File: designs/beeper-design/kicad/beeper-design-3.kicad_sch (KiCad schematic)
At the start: 30 parts, among them U12 DRV2605YZFR, U13 CSD75207W15, U3 BQ51003YFPR

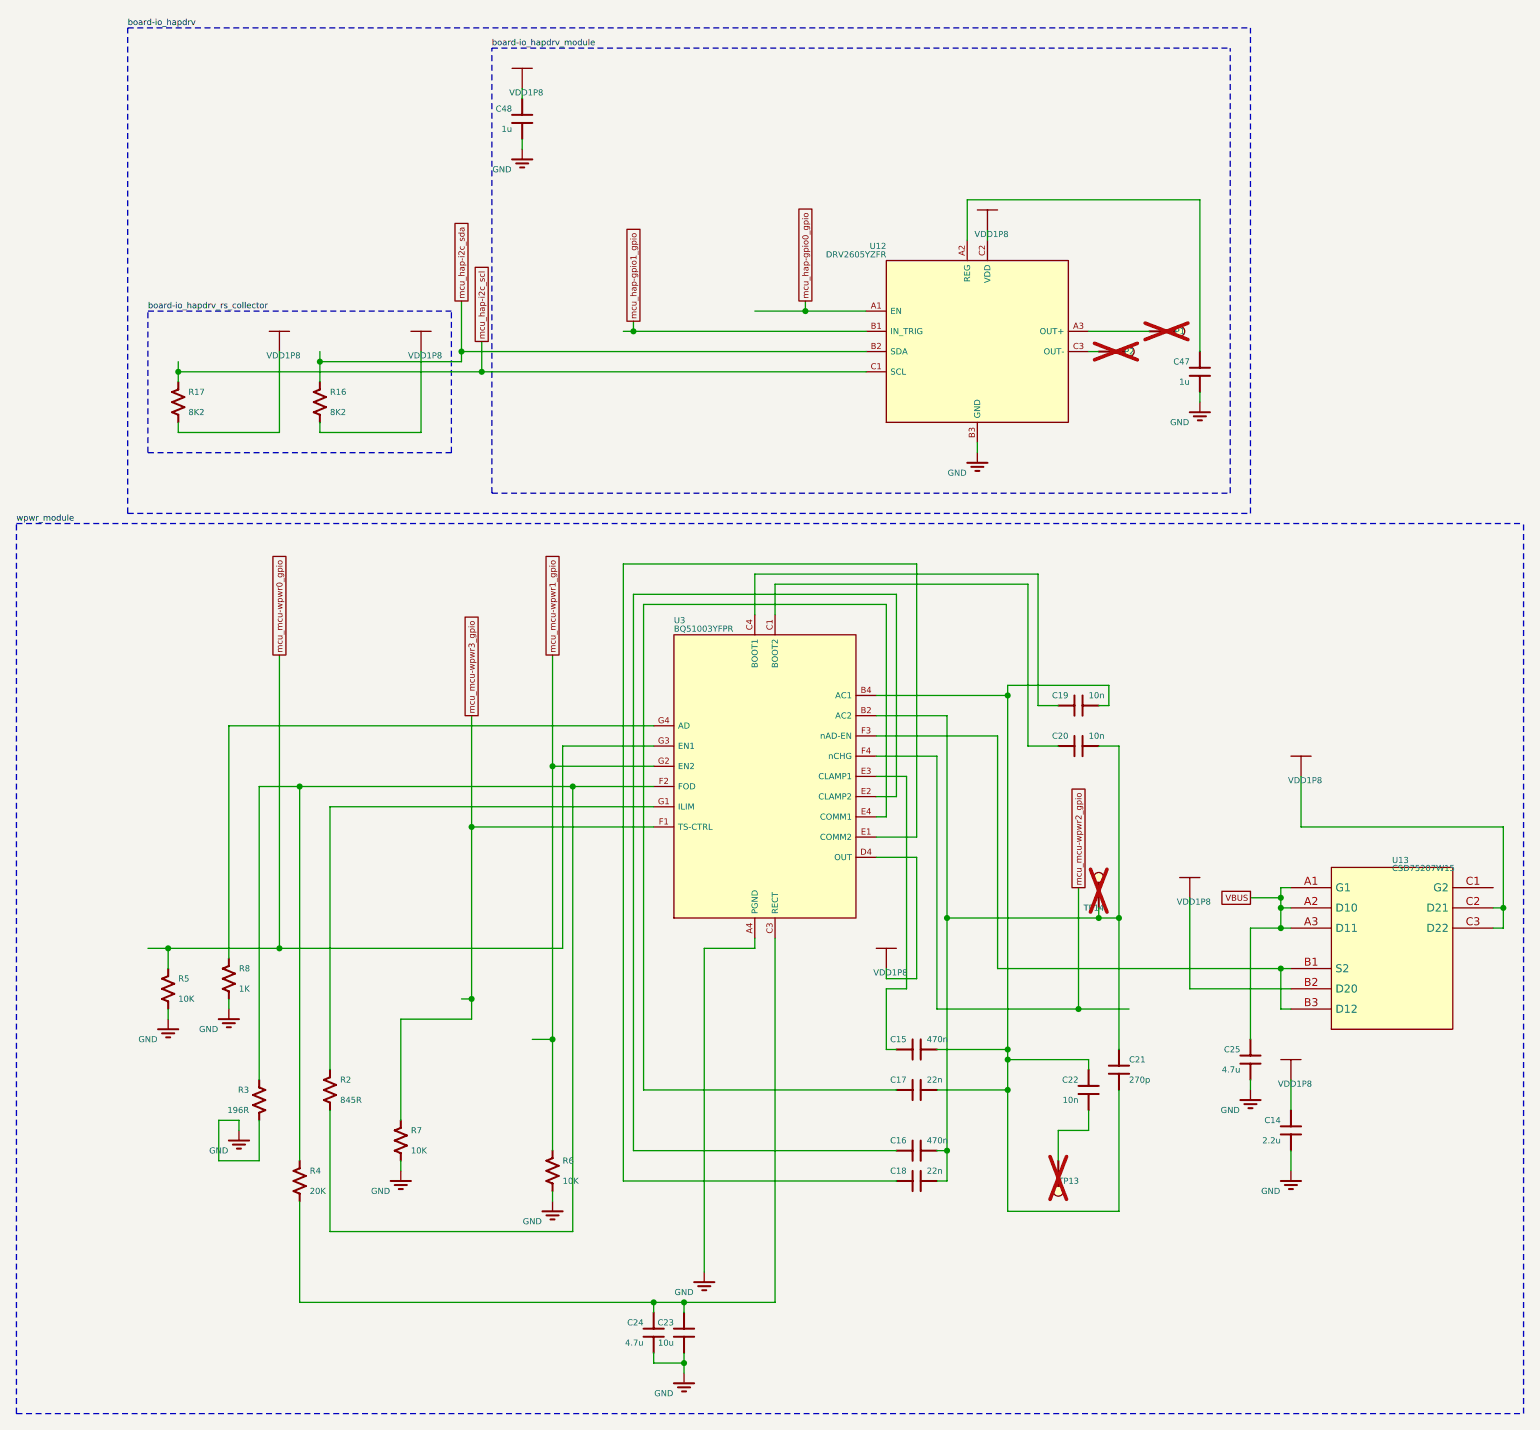
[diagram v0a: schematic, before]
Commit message: exported yet again
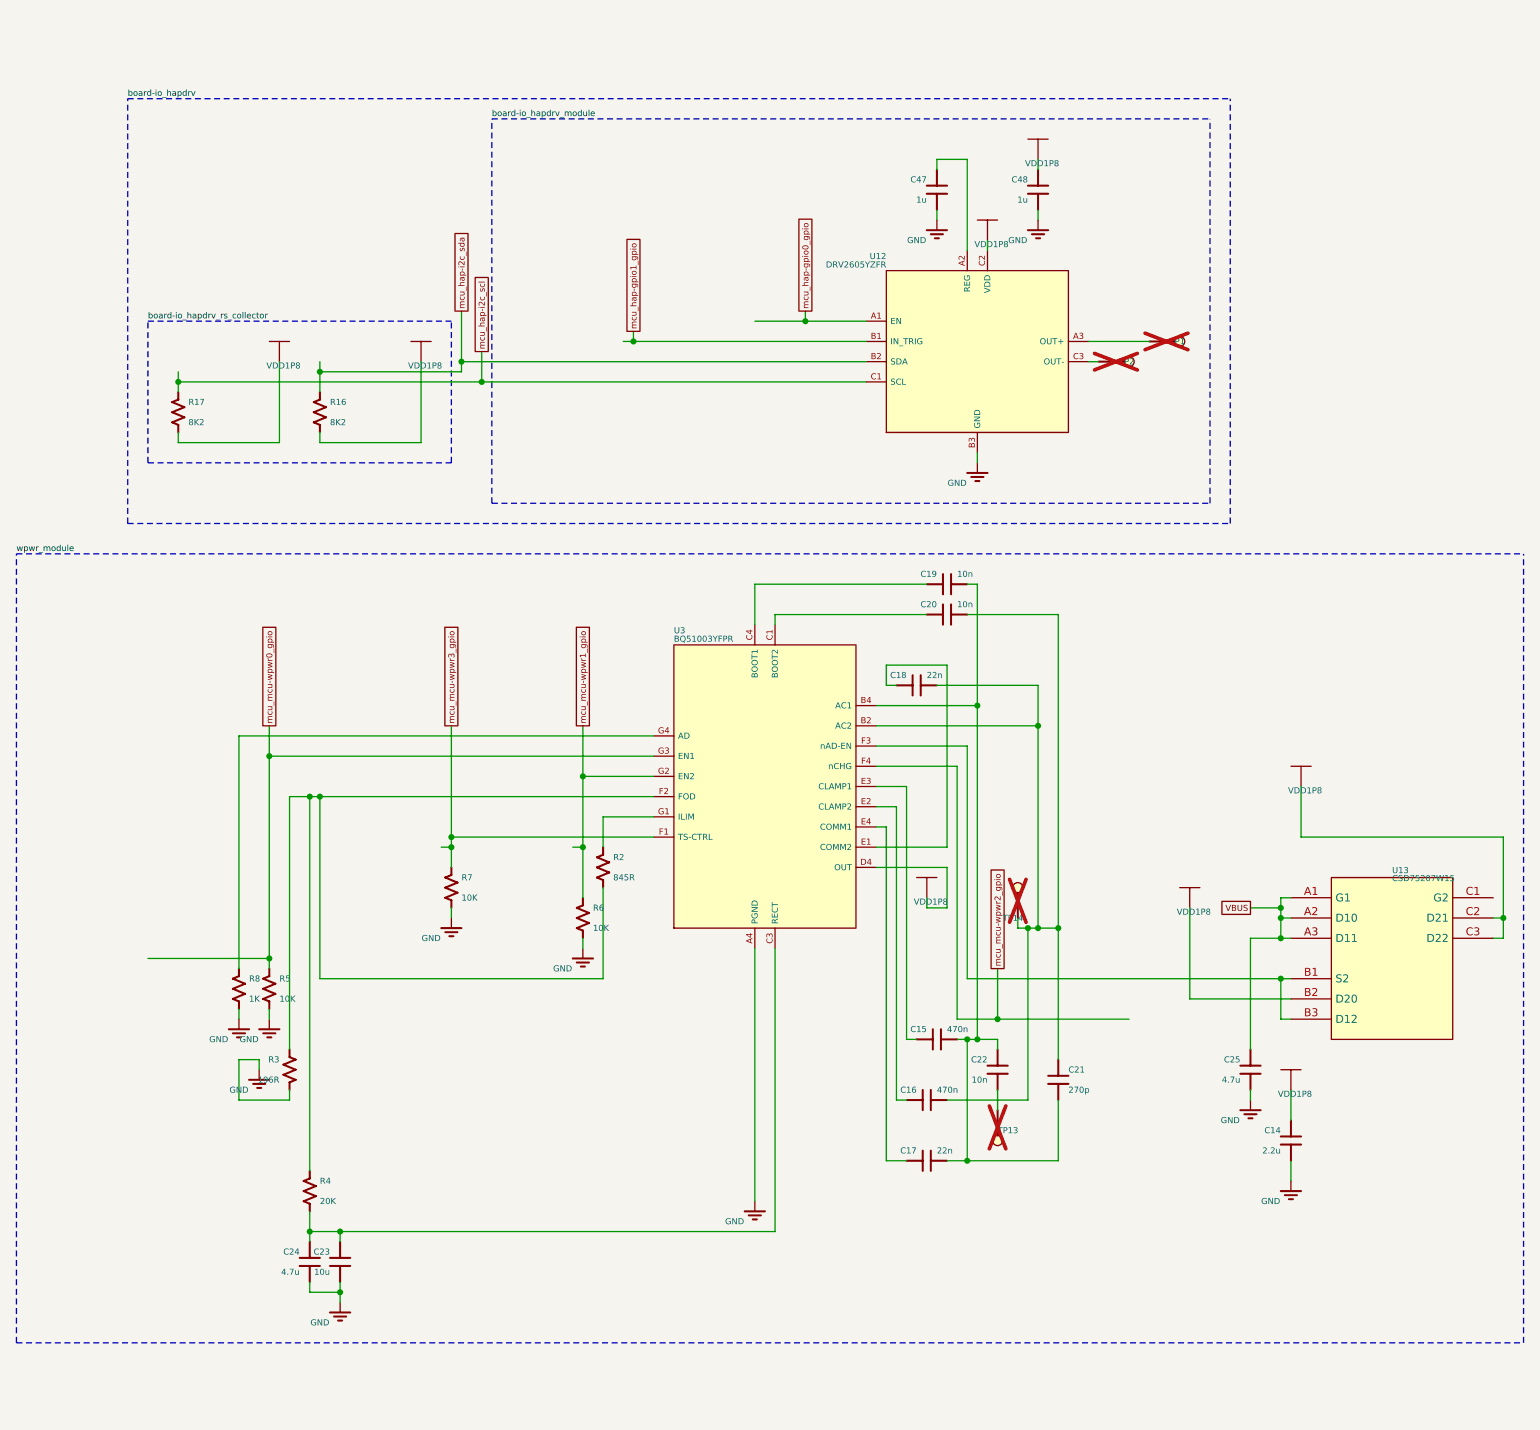
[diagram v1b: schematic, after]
